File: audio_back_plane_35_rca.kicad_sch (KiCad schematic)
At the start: 166 parts, among them IC1 74HCT2G125DC,125, IC3 TMUX4052BQBR, IC5 TMUX4053DYYR, J1 PJRAS2X1S01X, J2 PJRAS2X1S01X, J3 Conn_01x01_Pin, J4 jumper, J5 jumper, J6 jumper, J7 jumper, J8 jumper, J9 jumper, SW1 RotaryEncoder_Switch_MP, SW2 TL1105WF160Q - 3.15mm actuator, SW3 TL1105WF160Q - 3.15mm actuator, SW4 TL1105WF160Q - 3.15mm actuator, SW5 SW_SPST, SW6 TL1105WF160Q - 3.15mm actuator, SW7 SW_SPST, SW8 SW_SPST, U1 Teensy 4.1 - DEVKIT, U10 SN74LVC1T45DBV, U11 SN74LVC1T45DBV, U12 SN74LVC1T45DBV, U13 SN74LVC1T45DBV, U14 Single Buffer - 74LVC1G125GV,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, U17 Single Buffer - 74LVC1G125GV,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, U18 Single Buffer - 74LVC1G125GV,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, U19 Single Buffer - 74LVC1G125GV,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, U2 ESP32-DevKitC - DEVKIT, U20 Single Buffer - 74LVC1G125GV,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, U21 SN74LVC2G125DCTR, U22 SN74LVC2G125DCTR, U23 SN74LVC2G125DCTR, U24 SN74LVC2G125DCTR, U3 SN74LVC245APW, U4 Single Buffer - 74LVC1G125GV,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, U5 Optoisolators - H11L1SM - 6-S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, U6 Dual Buffer - 74HCT2G17GW,125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, U7 Single Buffer - 74LVC1G125GV,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, U8 Single Buffer - 74LVC1G125GV,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, U9 SN74LVC1T45DBV

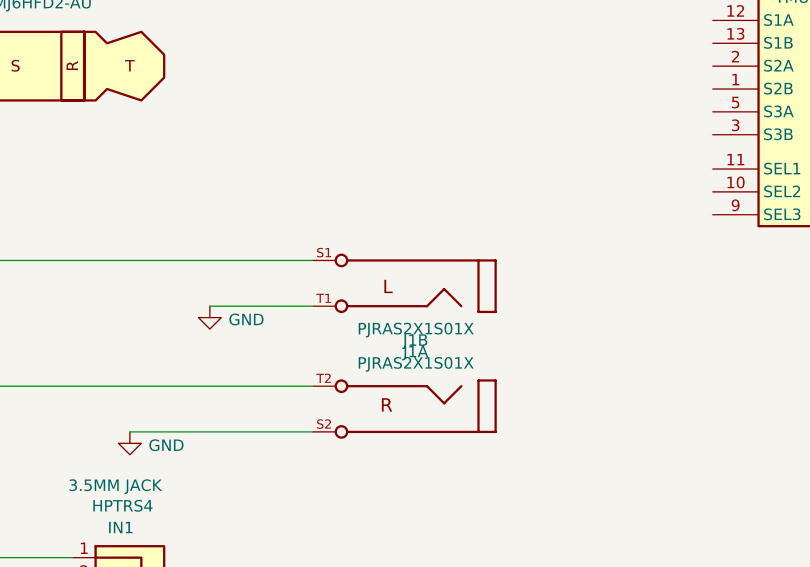
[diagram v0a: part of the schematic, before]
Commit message: update
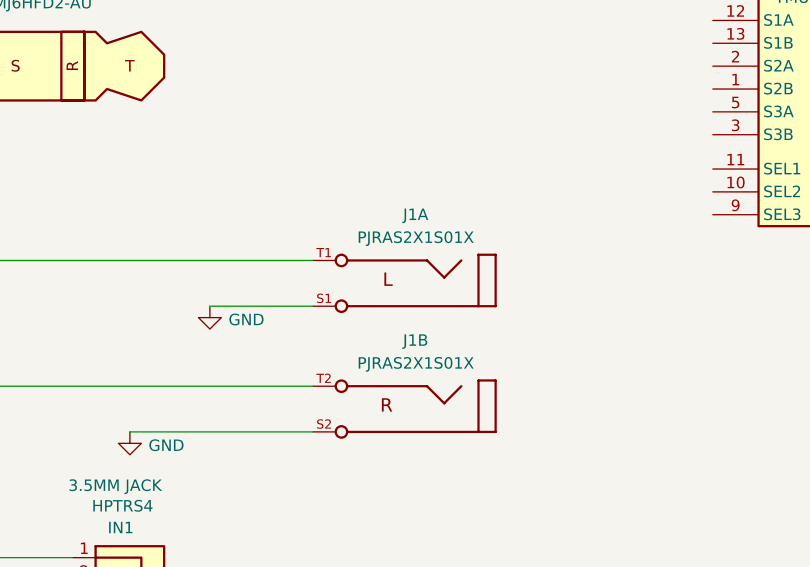
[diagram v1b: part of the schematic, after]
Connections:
- net GND: now also J1.S1; no longer J1.T1
- net at HPTRS4.3, J5.2: now also J1.T1; no longer J1.S1
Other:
- moved on the sheet: J1A
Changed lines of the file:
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@@
 	(symbol
 		(lib_id "PJRAS2X1S01X:PJRAS2X1S01X")
-		(at 566.42 662.94 180)
+		(at 566.42 662.94 0)
+		(mirror y)
 		(unit 1)
 		(exclude_from_sim no)
@@
 		(dnp no)
 		(property "Reference" "J1"
-			(at 566.4245 670.56 0)
+			(at 566.4245 655.32 0)
 			(effects
 				(font
@@
 		)
 		(property "Value" "PJRAS2X1S01X"
-			(at 566.4245 668.02 0)
+			(at 566.4245 657.86 0)
 			(effects
 				(font

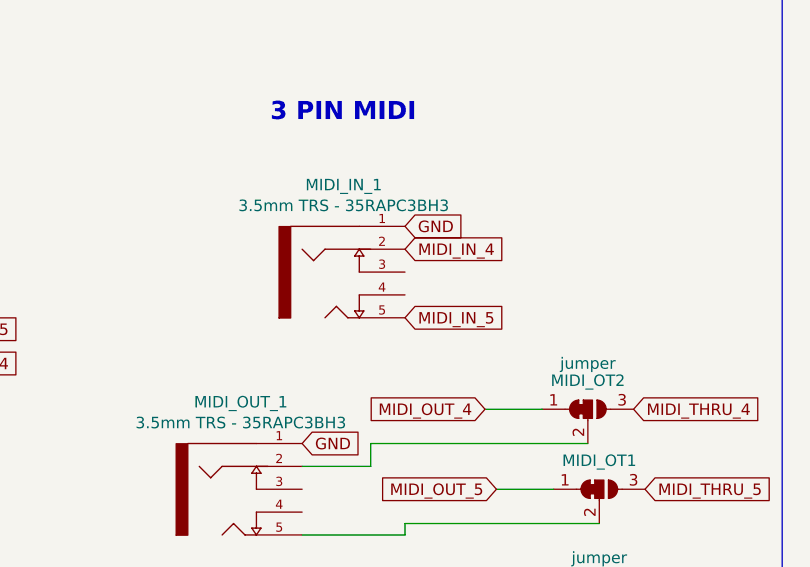
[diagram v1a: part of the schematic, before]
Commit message: update
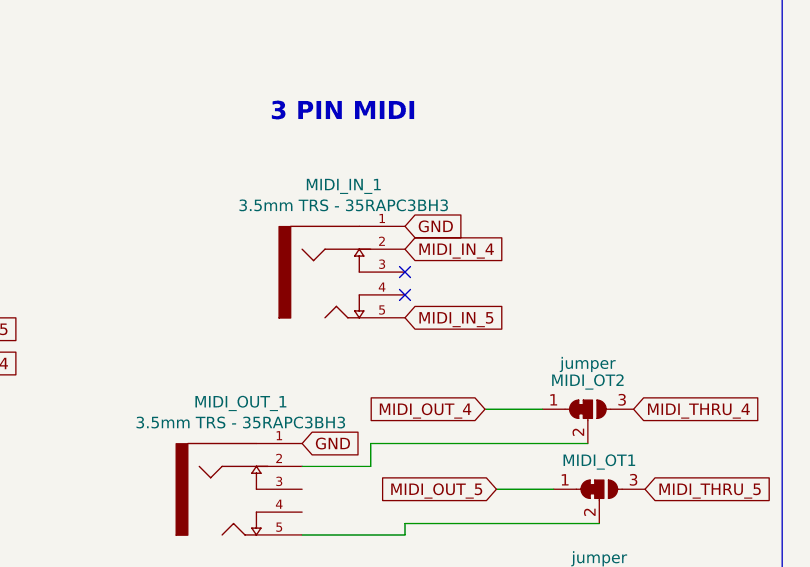
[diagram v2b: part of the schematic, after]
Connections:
- no-connect marks 13 -> 15
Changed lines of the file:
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@@
+	)
+	(no_connect
+		(at 1070.61 568.96)
+	)
+	(no_connect
+		(at 1070.61 571.5)
 	)
 	(no_connect
